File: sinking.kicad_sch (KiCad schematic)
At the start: 14 parts, among them Q1 Q_NPN_BCE, U1 LTV-817, U2 V7805-1000, U3 INA219AxD, U4 74HC14

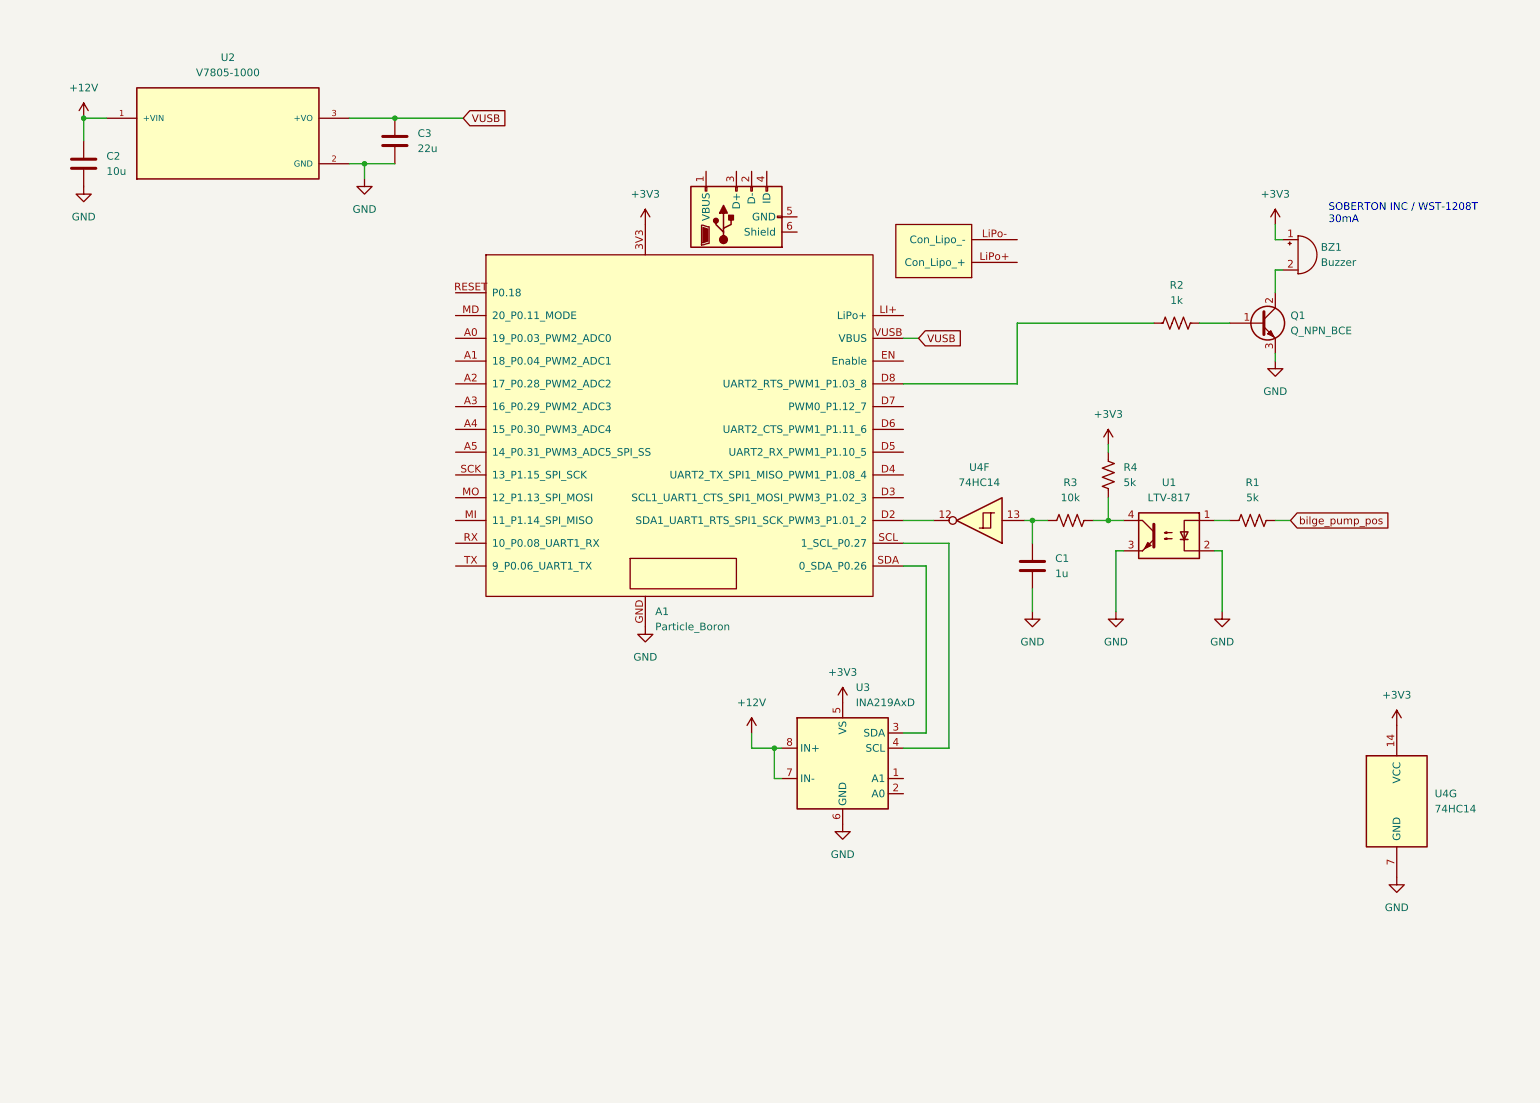
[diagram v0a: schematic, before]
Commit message: first layout
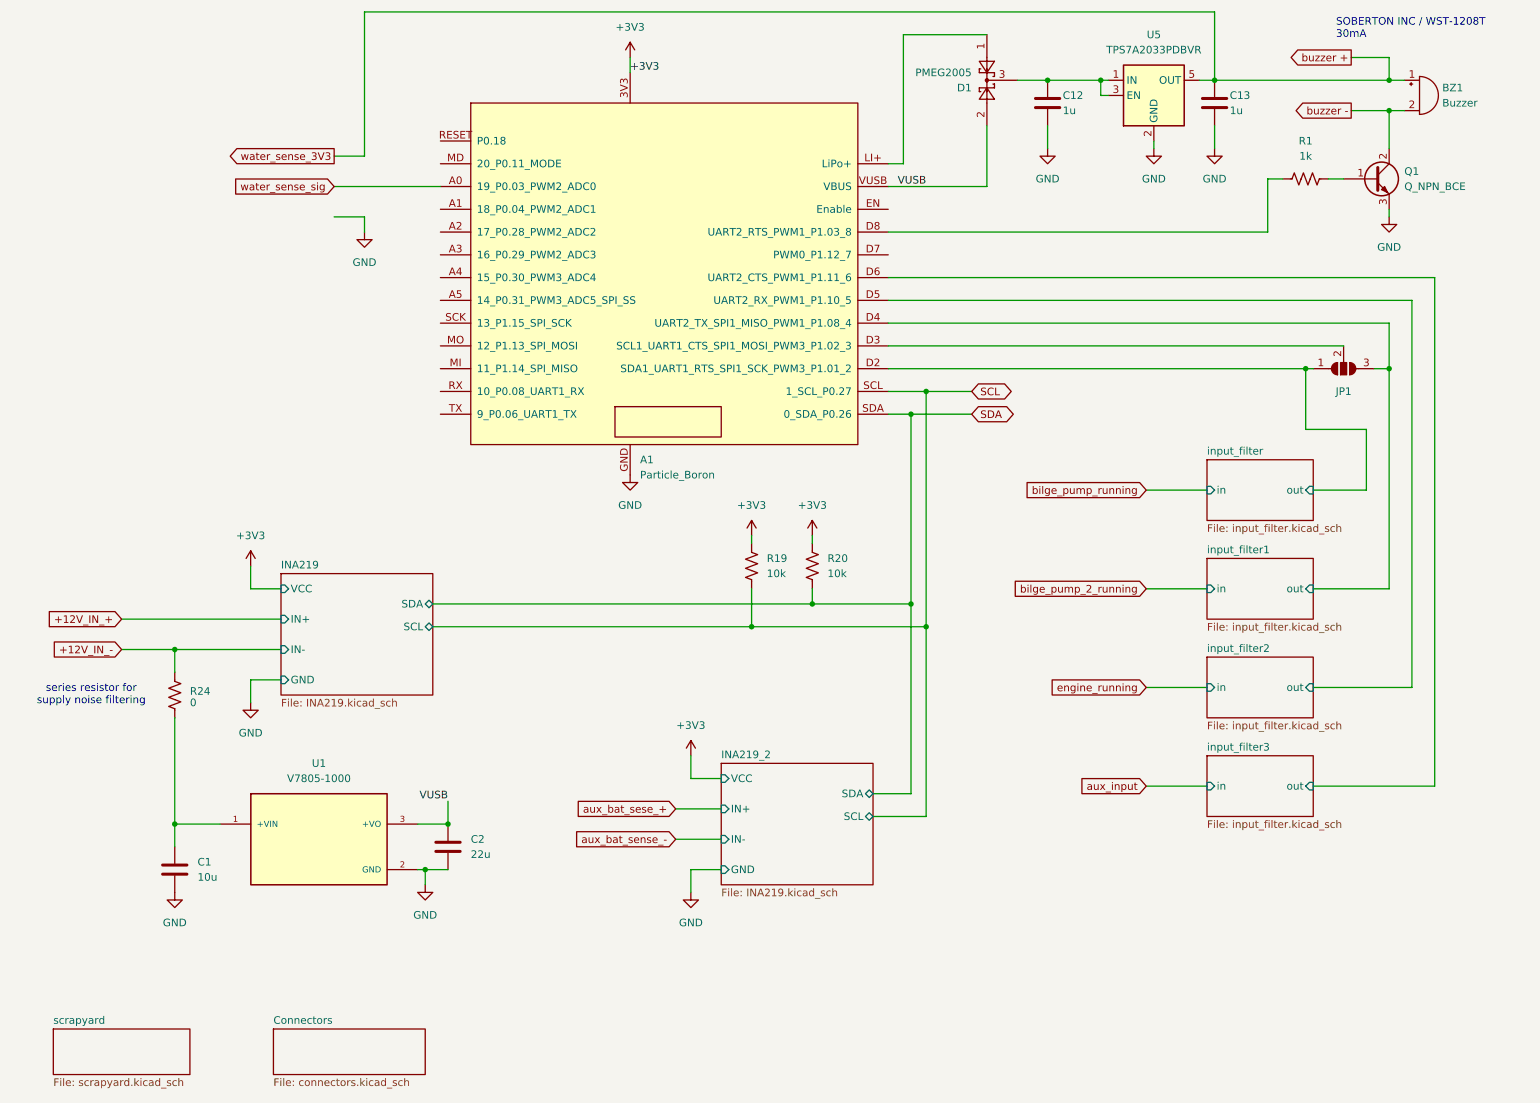
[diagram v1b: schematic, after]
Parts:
- removed C1: 1u, Capacitor_SMD:C_0805_2012Metric, symbol Device:C
- removed R1, R4: 5k, Resistor_SMD:R_0805_2012Metric, symbol Device:R_US
- removed R3: 10k, Resistor_SMD:R_0805_2012Metric, symbol Device:R_US
- removed U1: LTV-817, Package_DIP:DIP-4_W7.62mm, symbol Isolator:LTV-817
- removed U3: INA219AxD, Package_SO:SOIC-8_3.9x4.9mm_P1.27mm, symbol Sensor_Energy:INA219AxD
- removed U4: 74HC14, Package_DIP:DIP-14_W7.62mm, symbol 74xx:74HC14
- added C12, C13: 1u, Capacitor_SMD:C_0805_2012Metric, symbol Device:C
- added D1: PMEG2005, Package_TO_SOT_SMD:SOT-23_Handsoldering, symbol Diode:BAT54C
- added JP1: SolderJumper_3_Open, Jumper:SolderJumper-3_P2.0mm_Open_TrianglePad1.0x1.5mm, symbol Jumper:SolderJumper_3_Open
- added R19, R20: 10k, Resistor_SMD:R_0805_2012Metric, symbol Device:R_US
- added R24: 0, Resistor_SMD:R_1210_3225Metric_Pad1.30x2.65mm_HandSolder, symbol Device:R_US
- added U5: TPS7A2033PDBVR, Package_TO_SOT_SMD:SOT-23-5, symbol Regulator_Linear:TPS7A0533PDBV
- A1: footprint boron:Boron -> libs:Boron; symbol particle:Particle_Boron -> particle_lib:Particle_Boron
- renumbered C2 to C1, C3 to C2, R2 to R1, U2 to U1
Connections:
- net +3V3: now also R19.2, R20.2; no longer BZ1.1 (+)
- net GND: now also C12.2, C13.2, U5.2 (GND)
- net VUSB: now also D1.2
- net buzzer -: now reaches BZ1.2 (-), Q1.2 (C)
- net water_sense_sig: now reaches A1.A0 (19_P0.03_PWM2_ADC0)
- net input_filter/out: now reaches A1.D2 (SDA1_UART1_RTS_SPI1_SCK_PWM3_P1.01_2)
- net input_filter/out: now also JP1.1 (A)
- net at A1.D3 (SCL1_UART1_CTS_SPI1_MOSI_PWM3_P1.02_3): now also JP1.2 (C)
- net input_filter1/out: now reaches A1.D4 (UART2_TX_SPI1_MISO_PWM1_P1.08_4)
- net input_filter1/out: now also JP1.3 (B)
- net input_filter2/out: now reaches A1.D5 (UART2_RX_PWM1_P1.10_5)
- net input_filter3/out: now reaches A1.D6 (UART2_CTS_PWM1_P1.11_6)
- net at A1.LI+ (LiPo+): now also D1.1
- net SCL: now reaches A1.SCL (1_SCL_P0.27)
- net SCL: now also R19.1
- net SDA: now reaches A1.SDA (0_SDA_P0.26)
- net SDA: now also R20.1
- net +12V: no longer names the net of C1.1, U1.1 (+VIN)
- net +12V: now also R24.2
- new net: C12.1, D1.3, U5.1 (IN), U5.3 (EN)
- new net +12V_IN_-: R24.1
- new net buzzer +: BZ1.1 (+), C13.1, U5.5 (OUT)
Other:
- added sheet Connectors (connectors.kicad_sch)
- added sheet INA219 (INA219.kicad_sch)
- added sheet INA219_2 (INA219.kicad_sch)
- added sheet input_filter (input_filter.kicad_sch)
- added sheet input_filter1 (input_filter.kicad_sch)
- added sheet input_filter2 (input_filter.kicad_sch)
- added sheet input_filter3 (input_filter.kicad_sch)
- added sheet scrapyard (scrapyard.kicad_sch)
- note added: "series resistor for supply noise filtering"
- moved on the sheet: BZ1, C1, C2, Q1, R1, U1
